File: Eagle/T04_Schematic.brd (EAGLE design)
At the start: 40.6 x 63.5 mm, 29 parts

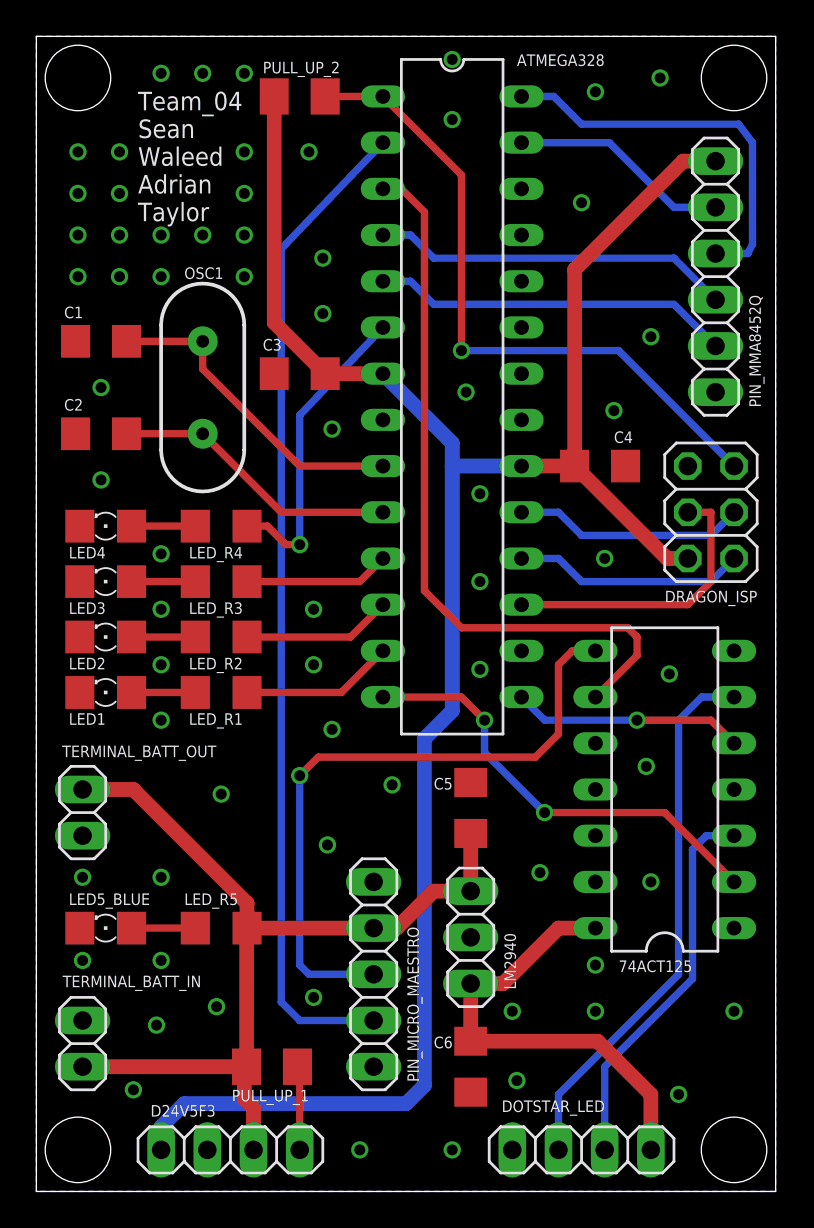
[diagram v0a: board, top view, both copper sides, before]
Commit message: Minor Tweaks and Fixes
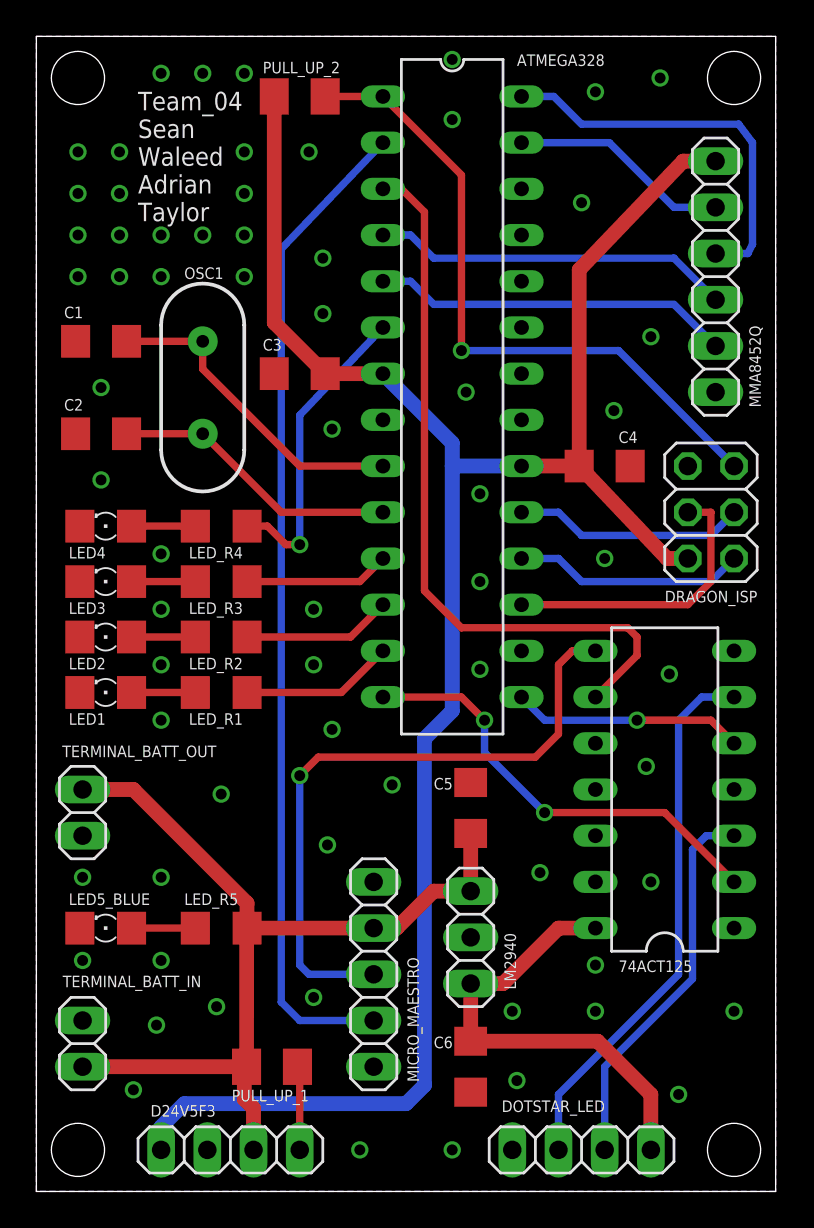
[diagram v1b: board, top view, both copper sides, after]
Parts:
- moved C4 0.25 mm to (31.2, 39.9)
- renumbered PIN_MICRO_MAESTRO to MICRO_MAESTRO, PIN_MMA8452Q to MMA8452Q
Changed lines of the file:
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@@
 <layer number="17" name="Pads" color="2" fill="1" visible="yes" active="yes"/>
 <layer number="18" name="Vias" color="2" fill="1" visible="yes" active="yes"/>
-<layer number="19" name="Unrouted" color="6" fill="1" visible="yes" active="yes"/>
+<layer number="19" name="Unrouted" color="6" fill="1" visible="no" active="yes"/>
 <layer number="20" name="Dimension" color="15" fill="1" visible="yes" active="yes"/>
 <layer number="21" name="tPlace" color="7" fill="1" visible="yes" active="yes"/>
@@
 <layer number="45" name="Holes" color="7" fill="1" visible="yes" active="yes"/>
 <layer number="46" name="Milling" color="3" fill="1" visible="no" active="yes"/>
-<layer number="47" name="Measures" color="7" fill="1" visible="yes" active="yes"/>
-<layer number="48" name="Document" color="7" fill="1" visible="yes" active="yes"/>
-<layer number="49" name="Reference" color="7" fill="1" visible="yes" active="yes"/>
+<layer number="47" name="Measures" color="7" fill="1" visible="no" active="yes"/>
+<layer number="48" name="Document" color="7" fill="1" visible="no" active="yes"/>
+<layer number="49" name="Reference" color="7" fill="1" visible="no" active="yes"/>
 <layer number="50" name="dxf" color="7" fill="1" visible="no" active="no"/>
 <layer number="51" name="tDocu" color="7" fill="1" visible="yes" active="yes"/>
@@
 Adrian
 Taylor</text>
-<hole x="2.286" y="61.214" drill="3.6"/>
-<hole x="38.354" y="61.214" drill="3.6"/>
-<hole x="2.286" y="2.286" drill="3.6"/>
-<hole x="38.354" y="2.286" drill="3.6"/>
+<hole x="2.286" y="61.214" drill="2.921"/>
+<hole x="38.354" y="61.214" drill="2.921"/>
+<hole x="2.286" y="2.286" drill="2.921"/>
+<hole x="38.354" y="2.286" drill="2.921"/>
 </plain>
 <attributes>
@@
 <attribute name="VALUE" x="34.925" y="12.573" size="0.6096" layer="27" ratio="10" rot="R180"/>
 </element>
-<element name="C4" library="rcl" package="C1206" value="100 nF" x="30.988" y="39.878" smashed="yes">
-<attribute name="NAME" x="31.75" y="41.148" size="0.635" layer="25"/>
-<attribute name="VALUE" x="28.448" y="42.418" size="0.6096" layer="27"/>
+<element name="C4" library="rcl" package="C1206" value="100 nF" x="31.242" y="39.878" smashed="yes">
+<attribute name="NAME" x="32.004" y="41.148" size="0.635" layer="25"/>
+<attribute name="VALUE" x="28.702" y="42.418" size="0.6096" layer="27"/>
 </element>
 <element name="C3" library="rcl" package="C1206" value="100 nF" x="14.478" y="44.958" smashed="yes" rot="R180">
@@
 <attribute name="VALUE" x="11.43" y="17.018" size="1.27" layer="27" rot="R180"/>
 </element>
-<element name="PIN_MICRO_MAESTRO" library="pinhead" package="1X05" value="1x5" x="18.542" y="11.938" smashed="yes" rot="R270">
+<element name="MICRO_MAESTRO" library="pinhead" package="1X05" value="1x5" x="18.542" y="11.938" smashed="yes" rot="R270">
 <attribute name="NAME" x="21.0312" y="6.0198" size="0.635" layer="25" ratio="10" rot="R90"/>
 </element>
-<element name="PIN_MMA8452Q" library="pinhead" package="1X06" value="1x6" x="37.338" y="50.292" smashed="yes" rot="R270">
+<element name="MMA8452Q" library="pinhead" package="1X06" value="1x6" x="37.338" y="50.292" smashed="yes" rot="R270">
 <attribute name="NAME" x="39.8272" y="43.1038" size="0.635" layer="25" ratio="10" rot="R90"/>
 </element>
@@
 <contactref element="ATMEGA328" pad="8"/>
 <contactref element="TERMINAL_BATT_IN" pad="1"/>
-<contactref element="PIN_MMA8452Q" pad="6"/>
+<contactref element="MMA8452Q" pad="6"/>
 <contactref element="C4" pad="2"/>
 <contactref element="C3" pad="2"/>
@@
 <contactref element="D24V5F3" pad="3"/>
 <contactref element="TERMINAL_BATT_OUT" pad="2"/>
-<contactref element="PIN_MICRO_MAESTRO" pad="1"/>
+<contactref element="MICRO_MAESTRO" pad="1"/>
 <contactref element="LED5_BLUE" pad="C"/>
 <contactref element="C1" pad="2"/>
@@
 <contactref element="C3" pad="1"/>
 <contactref element="ATMEGA328" pad="7"/>
-<contactref element="PIN_MMA8452Q" pad="1"/>
+<contactref element="MMA8452Q" pad="1"/>
 <contactref element="DRAGON_ISP" pad="2"/>
 <wire x1="21.336" y1="24.892" x2="22.86" y2="26.416" width="0.8128" layer="16"/>
@@
 <wire x1="15.878" y1="44.958" x2="13.078" y2="47.758" width="0.8128" layer="1"/>
 <wire x1="13.078" y1="47.758" x2="13.078" y2="60.198" width="0.8128" layer="1"/>
-<wire x1="26.67" y1="39.878" x2="29.588" y2="39.878" width="0.8128" layer="1"/>
-<wire x1="29.588" y1="39.878" x2="34.668" y2="34.798" width="0.8128" layer="1"/>
+<wire x1="26.67" y1="39.878" x2="29.842" y2="39.878" width="0.8128" layer="1"/>
+<wire x1="29.842" y1="39.878" x2="34.668" y2="34.798" width="0.8128" layer="1"/>
 <wire x1="34.668" y1="34.798" x2="35.814" y2="34.798" width="0.8128" layer="1"/>
-<wire x1="29.588" y1="39.878" x2="29.588" y2="50.67" width="0.8128" layer="1"/>
-<wire x1="29.588" y1="50.67" x2="35.56" y2="56.642" width="0.8128" layer="1"/>
+<wire x1="29.842" y1="39.878" x2="29.842" y2="50.67" width="0.8128" layer="1"/>
+<wire x1="29.842" y1="50.67" x2="35.56" y2="56.642" width="0.8128" layer="1"/>
 <wire x1="35.56" y1="56.642" x2="37.338" y2="56.642" width="0.8128" layer="1"/>
 <wire x1="21.336" y1="5.842" x2="21.336" y2="24.892" width="0.8128" layer="16"/>
@@
 </signal>
 <signal name="SDA">
-<contactref element="PIN_MMA8452Q" pad="2"/>
+<contactref element="MMA8452Q" pad="2"/>
 <contactref element="ATMEGA328" pad="27"/>
 <wire x1="26.67" y1="57.658" x2="31.496" y2="57.658" width="0.4064" layer="16"/>
@@
 </signal>
 <signal name="SCL">
-<contactref element="PIN_MMA8452Q" pad="3"/>
+<contactref element="MMA8452Q" pad="3"/>
 <contactref element="ATMEGA328" pad="28"/>
 <wire x1="37.338" y1="51.562" x2="39.116" y2="51.562" width="0.4064" layer="16"/>
@@
 </signal>
 <signal name="INT0">
-<contactref element="PIN_MMA8452Q" pad="4"/>
+<contactref element="MMA8452Q" pad="4"/>
 <contactref element="ATMEGA328" pad="4"/>
 <wire x1="37.338" y1="49.022" x2="35.052" y2="51.308" width="0.4064" layer="16"/>
@@
 <signal name="INT1">
 <contactref element="ATMEGA328" pad="5"/>
-<contactref element="PIN_MMA8452Q" pad="5"/>
+<contactref element="MMA8452Q" pad="5"/>
 <wire x1="37.338" y1="46.482" x2="35.052" y2="48.768" width="0.4064" layer="16"/>
 <wire x1="35.052" y1="48.768" x2="21.844" y2="48.768" width="0.4064" layer="16"/>
@@
 </signal>
 <signal name="RXD">
-<contactref element="PIN_MICRO_MAESTRO" pad="3"/>
+<contactref element="MICRO_MAESTRO" pad="3"/>
 <contactref element="74ACT125" pad="8"/>
 <wire x1="18.542" y1="11.938" x2="14.986" y2="11.938" width="0.4064" layer="16"/>
@@
 </signal>
 <signal name="SERVO_TXD">
-<contactref element="PIN_MICRO_MAESTRO" pad="4"/>
+<contactref element="MICRO_MAESTRO" pad="4"/>
 <contactref element="ATMEGA328" pad="2"/>
 <wire x1="19.05" y1="57.658" x2="13.462" y2="51.816" width="0.4064" layer="16"/>
@@
 <contactref element="D24V5F3" pad="2"/>
 <contactref element="PULL_UP_1" pad="2"/>
-<contactref element="PIN_MICRO_MAESTRO" pad="2"/>
+<contactref element="MICRO_MAESTRO" pad="2"/>
 <contactref element="LED_R5" pad="1"/>
 <contactref element="C5" pad="1"/>
